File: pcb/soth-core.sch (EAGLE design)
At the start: 19 parts, among them IC1 FT231X USB Converter, IC2 REG1117, IC3 TC7SZ125F, IC4 TC7SZ125F, U1 ATXMEGA32D4-AU, X1 5V/4A

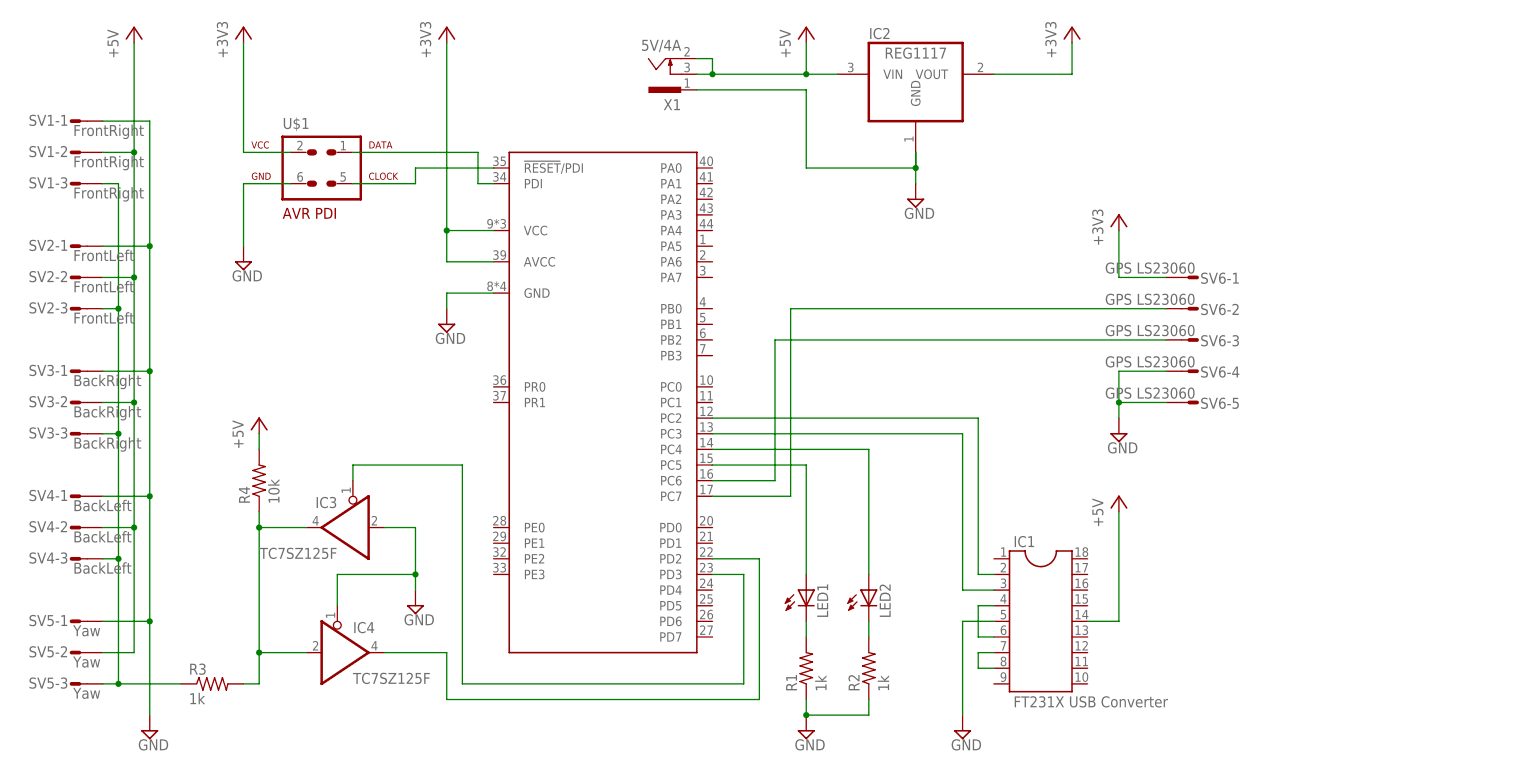
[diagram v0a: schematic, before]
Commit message: add i2c code
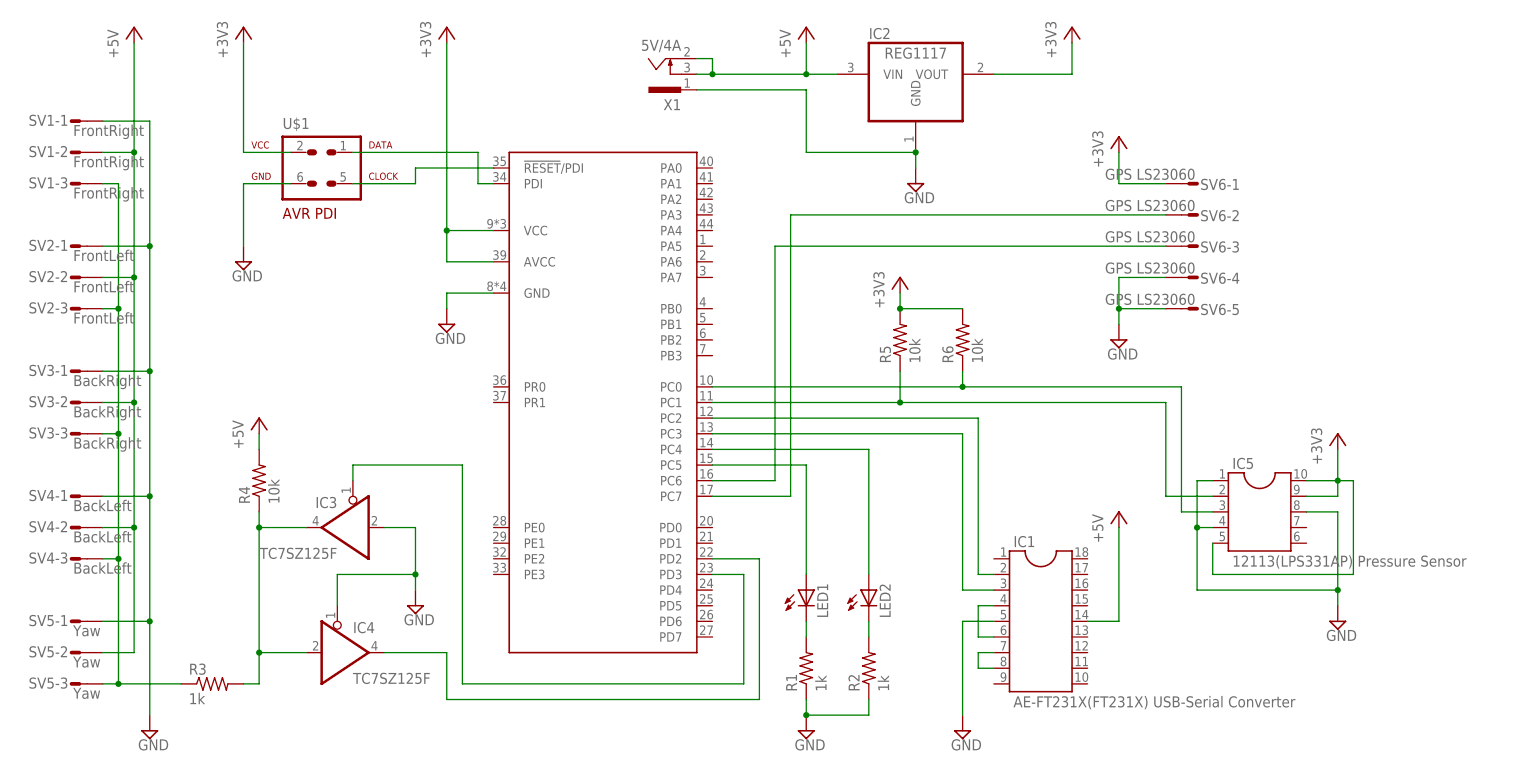
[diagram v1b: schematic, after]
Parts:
- added IC5: 12113(LPS331AP) Pressure Sensor, ic-package:DIL10
- added R5, R6: 10k, rcl:R-US_R0805
- IC1: value FT231X USB Converter -> AE-FT231X(FT231X) USB-Serial Converter
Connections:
- new net N$29: IC5.3, R6.1, U1.PC0
- new net N$32: IC5.2, R5.1, U1.PC1
- net +3V3: now also IC5.10, IC5.5, IC5.9, R5.2, R6.2
- net GND: now also IC5.1, IC5.4, IC5.8
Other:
- moved on the sheet: SV6-1, SV6-2, SV6-3, SV6-4, SV6-5
